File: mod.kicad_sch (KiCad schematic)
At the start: 5 parts, among them Q4 MMBF4391, SW2 SW_DPST, U6 TL074, U7 TL072, U8 LM13700

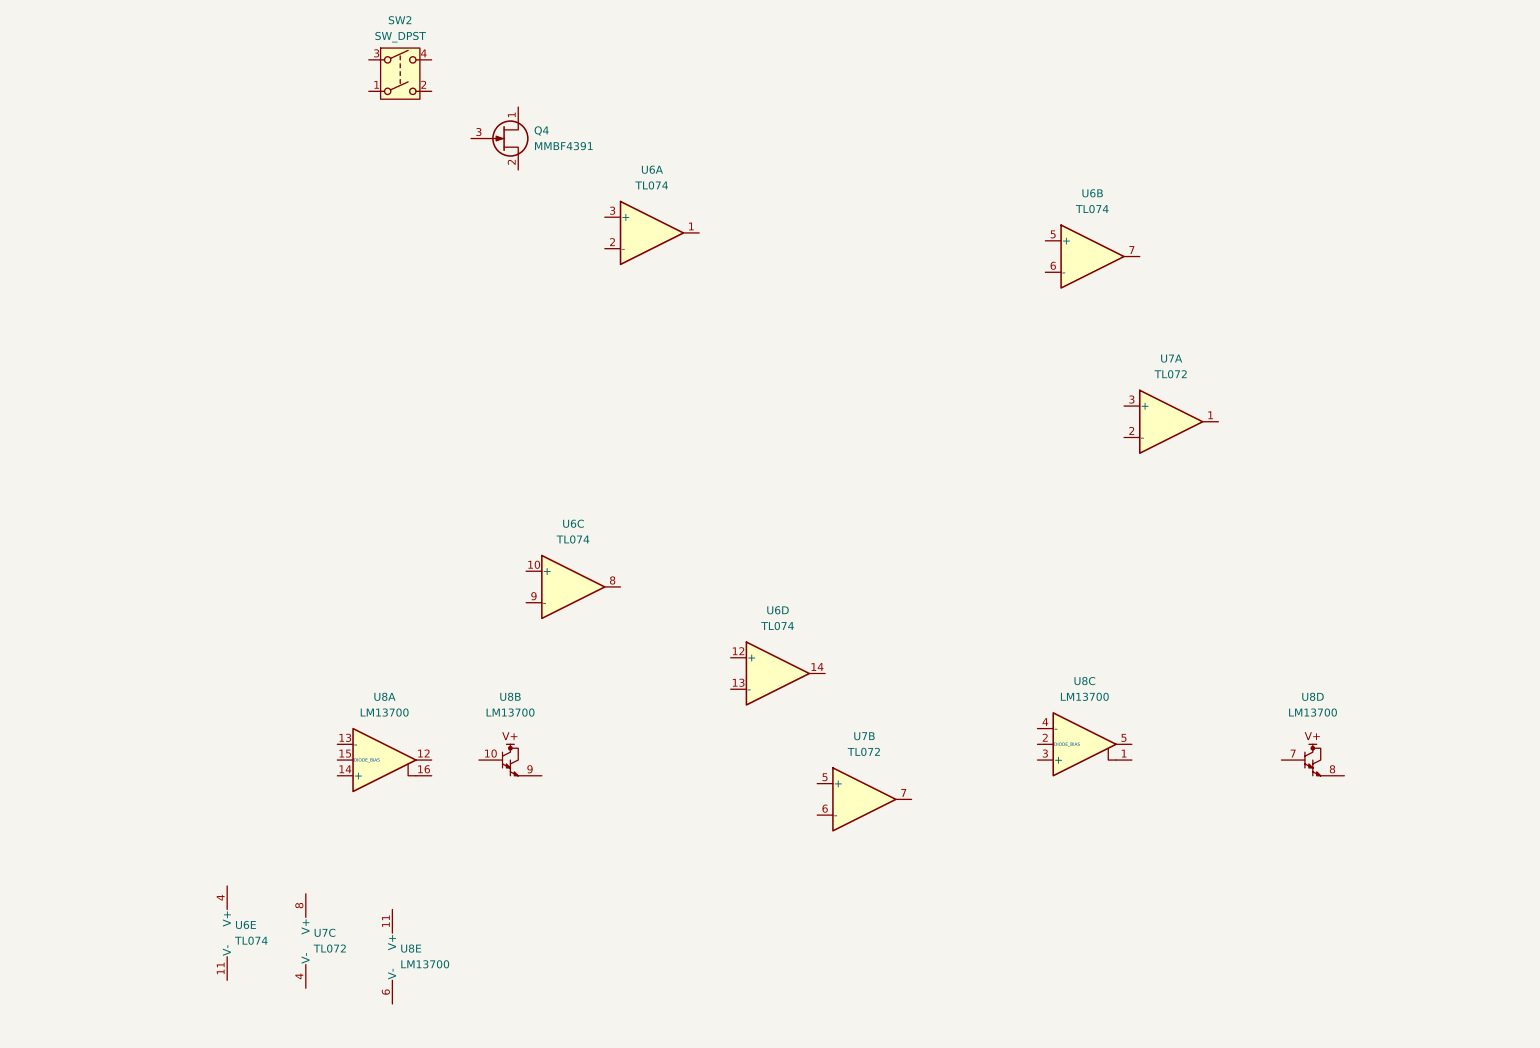
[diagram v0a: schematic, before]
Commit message: Finish schematic for modulation
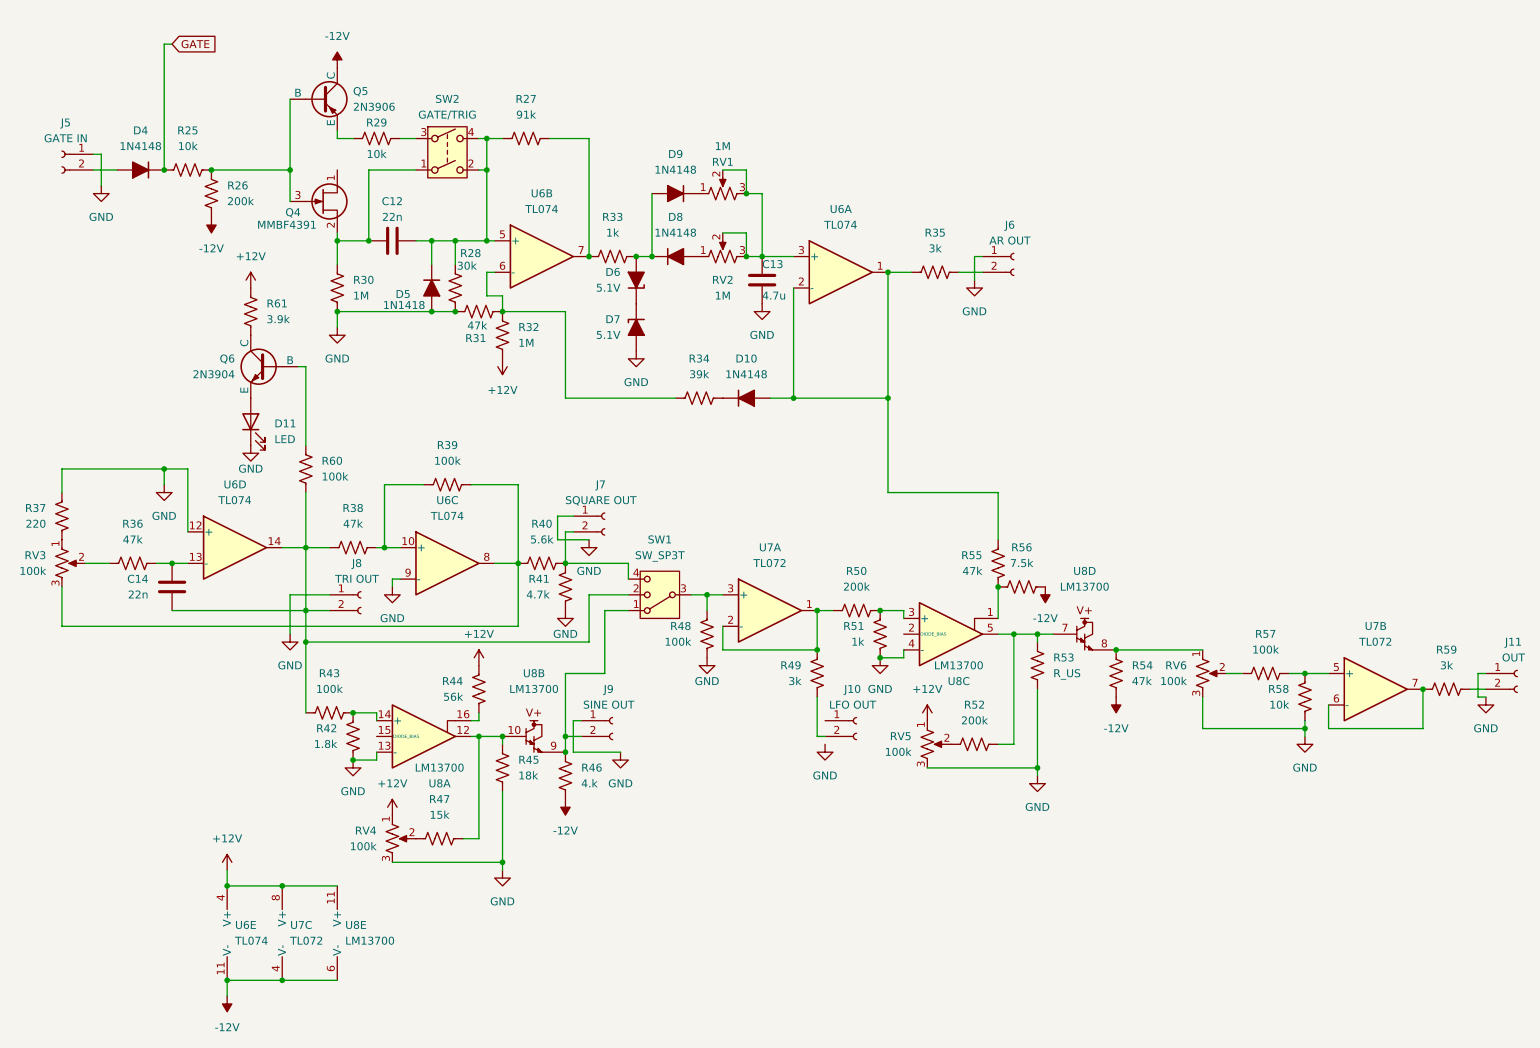
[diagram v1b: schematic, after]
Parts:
- added C12, C14: 22n, symbol Device:C
- added C13: 4.7u, symbol Device:C
- added D10, D4, D8, D9: 1N4148, symbol Device:D_Filled
- added D11: LED, symbol Device:LED
- added D5: 1N1418, symbol Device:D_Filled
- added D6, D7: 5.1V, symbol Device:D_Zener_Filled
- added J10: LFO OUT, symbol Connector:Conn_01x02_Socket
- added J11: OUT, symbol Connector:Conn_01x02_Socket
- added J5: GATE IN, symbol Connector:Conn_01x02_Socket
- added J6: AR OUT, symbol Connector:Conn_01x02_Socket
- added J7: SQUARE OUT, symbol Connector:Conn_01x02_Socket
- added J8: TRI OUT, symbol Connector:Conn_01x02_Socket
- added J9: SINE OUT, symbol Connector:Conn_01x02_Socket
- added Q5: 2N3906, symbol Simulation_SPICE:PNP
- added Q6: 2N3904, symbol Simulation_SPICE:NPN
- added R25, R29, R58: 10k, symbol Device:R_US
- added R26, R50, R52: 200k, symbol Device:R_US
- added R27: 91k, symbol Device:R_US
- added R28: 30k, symbol Device:R_US
- added R30, R32: 1M, symbol Device:R_US
- added R31, R36, R38, R54, R55: 47k, symbol Device:R_US
- added R33, R51: 1k, symbol Device:R_US
- added R34: 39k, symbol Device:R_US
- added R35, R49, R59: 3k, symbol Device:R_US
- added R37: 220, symbol Device:R_US
- added R39, R43, R48, R57, R60: 100k, symbol Device:R_US
- added R40: 5.6k, symbol Device:R_US
- added R41: 4.7k, symbol Device:R_US
- added R42: 1.8k, symbol Device:R_US
- added R44: 56k, symbol Device:R_US
- added R45: 18k, symbol Device:R_US
- added R46: 4.k, symbol Device:R_US
- added R47: 15k, symbol Device:R_US
- added R53: R_US, symbol Device:R_US
- added R56: 7.5k, symbol Device:R_US
- added R61: 3.9k, symbol Device:R_US
- added RV1, RV2: 1M, symbol Device:R_Potentiometer_US
- added RV3, RV4, RV5, RV6: 100k, symbol Device:R_Potentiometer_US
- added SW1: SW_SP3T, symbol Switch:SW_SP3T
- SW2: value SW_DPST -> GATE/TRIG
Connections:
- net GND: now reaches U6.12 (+)
- net GND: now also U6.9 (-), U8.13 (-), U8.4 (-), C13.2, D11.1 (K), D5.2 (A), D7.2 (A), J11.1 (Pin_1), J5.1 (Pin_1), J6.1 (Pin_1), J7.1 (Pin_1), J8.1 (Pin_1), J9.1 (Pin_1), R28.1, R30.2, R31.1, R37.2, R41.1, R42.1, R45.1, R48.1, R51.1, R53.1, R58.1, RV4.3, RV5.3, RV6.3
- net at U6.13 (-): now also C14.1, R36.2
- net at U6.14: now also C14.2, J8.2 (Pin_2), R38.1, R43.1, R60.2, SW1.2
- net at U8.7: now also U8.5, R52.2, R53.2
- net at U8.8: now also R54.2, RV6.1
- net at Q4.2 (S): now also SW2.1, C12.1, R30.1
- net at Q4.3 (G): now also Q5.2 (B), R25.2, R26.2
- net at U7.1: now also U7.2 (-), R49.2, R50.1
- net at U7.3 (+): now also R48.2, SW1.3
- net -12V: now reaches U7.4 (V-)
- net -12V: now also U6.11 (V-), U8.6 (V-), Q5.1 (C), R26.1, R46.1, R54.1, R56.2
- net +12V: now reaches U7.8 (V+)
- net +12V: now also U6.4 (V+), U8.11 (V+), R32.2, R44.2, R61.1, RV4.1, RV5.1
- net at U8.1: now also R55.1, R56.1
- net at U8.3 (+): now also R50.2, R51.2
- net at SW2.2: now also SW2.4, U6.5 (+), C12.2, D5.1 (K), R27.1, R28.2
- net at SW2.3: now also R29.2
- net at U6.6 (-): now also R31.2, R32.1, R34.1
- net at U6.7: now also R27.2, R33.1
- net at U6.10 (+): now also R38.2, R39.1
- net at U6.8: now also R39.2, R40.1, RV3.3
- net at U8.12: now also U8.10, R45.2, R47.2
- net at U8.14 (+): now also R42.2, R43.2
- net at U8.16: now also R44.1
- net at U8.9: now also J9.2 (Pin_2), R46.2, SW1.1
- net at U6.1: now also U6.2 (-), D10.2 (A), R35.1, R55.2
- net at U6.3 (+): now also C13.1, RV1.2, RV1.3, RV2.2, RV2.3
- net at U7.5 (+): now also R57.2, R58.2
- net at U7.6 (-): now also U7.7, R59.1
- new net: R47.1, RV4.2
- new net: D10.1 (K), R34.2
- new net: R37.1, RV3.1
- new net: R36.1, RV3.2
- new net: D4.2 (A), J5.2 (Pin_2)
- new net: D6.2 (A), D8.1 (K), D9.2 (A), R33.2
- new net: D8.2 (A), RV2.1
- new net: D9.1 (K), RV1.1
- new net: Q6.2 (B), R60.1
- new net: J7.2 (Pin_2), R40.2, R41.2, SW1.4
- new net: Q6.1 (C), R61.2
- new net: D11.2 (A), Q6.3 (E)
- new net: R57.1, RV6.2
- new net: R52.1, RV5.2
- new net: J6.2 (Pin_2), R35.2
- new net: Q5.3 (E), R29.1
- new net: J10.2 (Pin_2), R49.1
- new net: J11.2 (Pin_2), R59.2
- new net: D6.1 (K), D7.1 (K)
- new net GATE: D4.1 (K), R25.1
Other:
- moved on the sheet: Q4, SW2, U6A, U6B, U6C, U6D, U7A, U7B, U7C, U8A, U8B, U8C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
